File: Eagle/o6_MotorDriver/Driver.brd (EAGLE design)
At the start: 160 x 100 mm, 13 parts, among them IC3 TINY13-20SSU

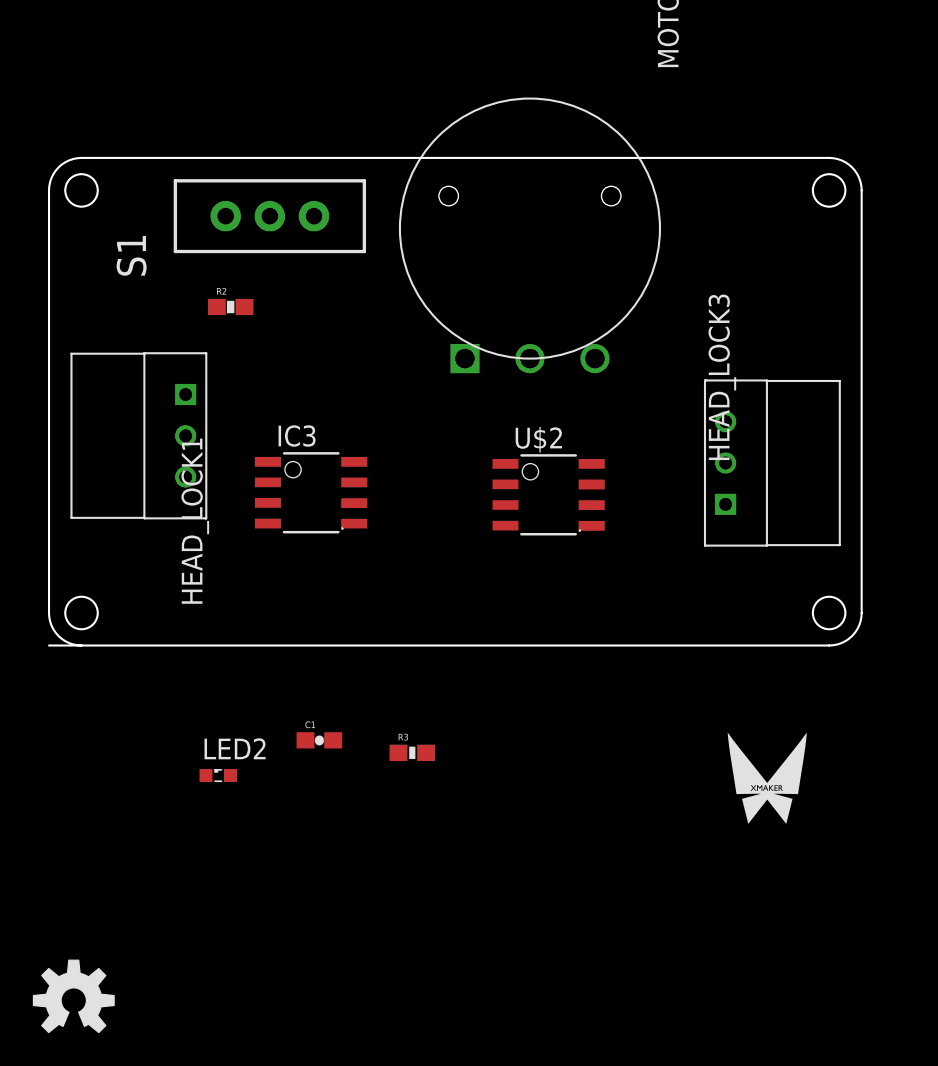
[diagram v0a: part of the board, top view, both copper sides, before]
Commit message: gxzz
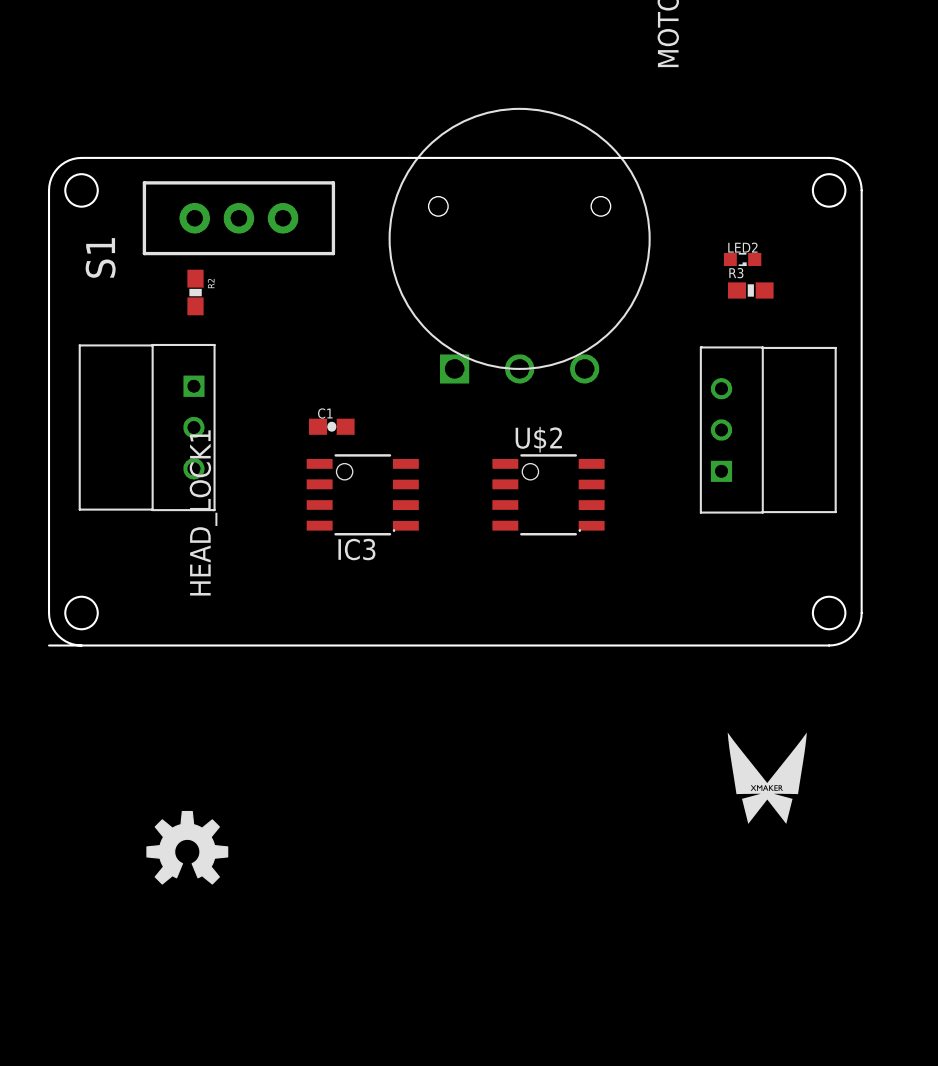
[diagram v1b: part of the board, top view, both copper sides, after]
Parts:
- moved LED2 45.3 mm to (43.7, -48.0), turned to 180 degrees
- moved R3 35.3 mm to (44.2, -49.9)
- moved C1 19.3 mm to (18.4, -58.3)
- moved U$8 11.5 mm to (9.53, -84.5)
- moved IC3 3.18 mm to (20.3, -62.5)
- moved R2 2.33 mm to (10.0, -50.0), turned to 270 degrees
- moved HEAD_LOCK3 2.05 mm to (42.4, -58.5)
- moved S1 1.91 mm to (12.7, -45.5)
- moved U$6 0.90 mm to (30.0, -54.7)
- moved HEAD_LOCK1 0.72 mm to (9.91, -58.3)
